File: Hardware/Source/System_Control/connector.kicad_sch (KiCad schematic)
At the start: 47 parts, among them J10 NTC_CONN, J11 NTC_CONN, J12 NTC_CONN, J13 NTC_CONN, J14 NTC_CONN, J15 NTC_CONN, J16 BAL_BAT_CONN2, J17 NTC_CONN, J18 NTC_CONN, J19 NTC_CONN, J20 NTC_CONN, J21 NTC_CONN, J22 NTC_CONN, J23 NTC_CONN, J24 NTC_CONN, J3 SIGNAL_CONN, J4 Conn_01x02_Socket, J5 FLASH_CONN, J6 Conn_01x02_Socket, J7 BAL_BAT_CONN1, J8 NTC_CONN, J9 NTC_CONN

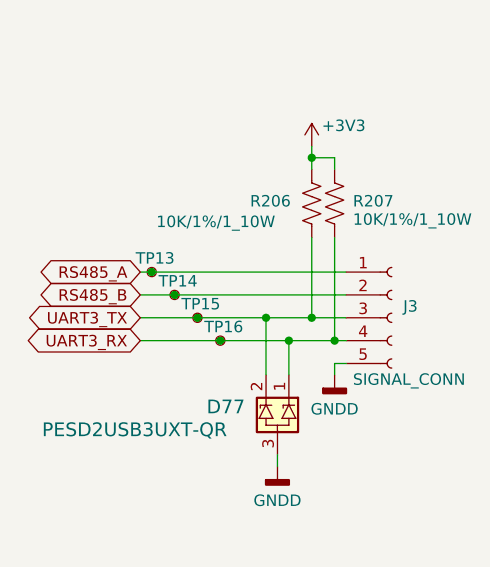
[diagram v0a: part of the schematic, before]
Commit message: pull
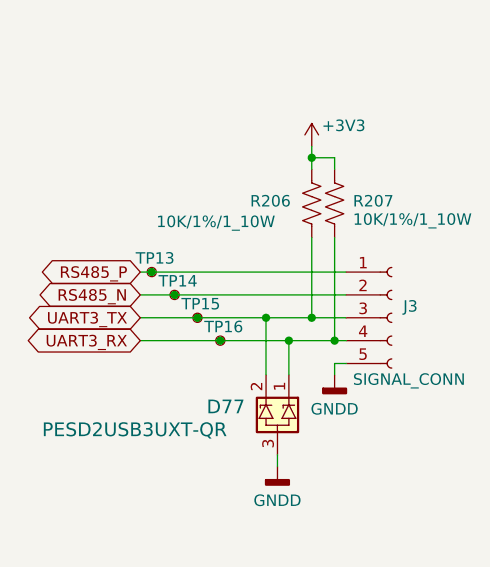
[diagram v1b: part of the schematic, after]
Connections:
- net RS485_A renamed RS485_P
- net RS485_B renamed RS485_N
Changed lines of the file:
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@@
 		)
 	)
-	(global_label "RS485_B"
+	(global_label "RS485_N"
 		(shape bidirectional)
 		(at 48.26 110.49 180)
@@
 		)
 		(property "Intersheetrefs" "${INTERSHEET_REFS}"
-			(at 35.8179 110.49 0)
+			(at 35.7574 110.49 0)
 			(effects
 				(font
@@
 		)
 	)
-	(global_label "RS485_A"
+	(global_label "RS485_P"
 		(shape bidirectional)
 		(at 48.26 107.95 180)
@@
 		)
 		(property "Intersheetrefs" "${INTERSHEET_REFS}"
-			(at 35.9993 107.95 0)
-			(effects
-				(font
+			(at 35.8179 107.95 0)
+			(effects
+				(font
